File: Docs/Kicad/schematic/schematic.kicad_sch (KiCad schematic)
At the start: 35 parts

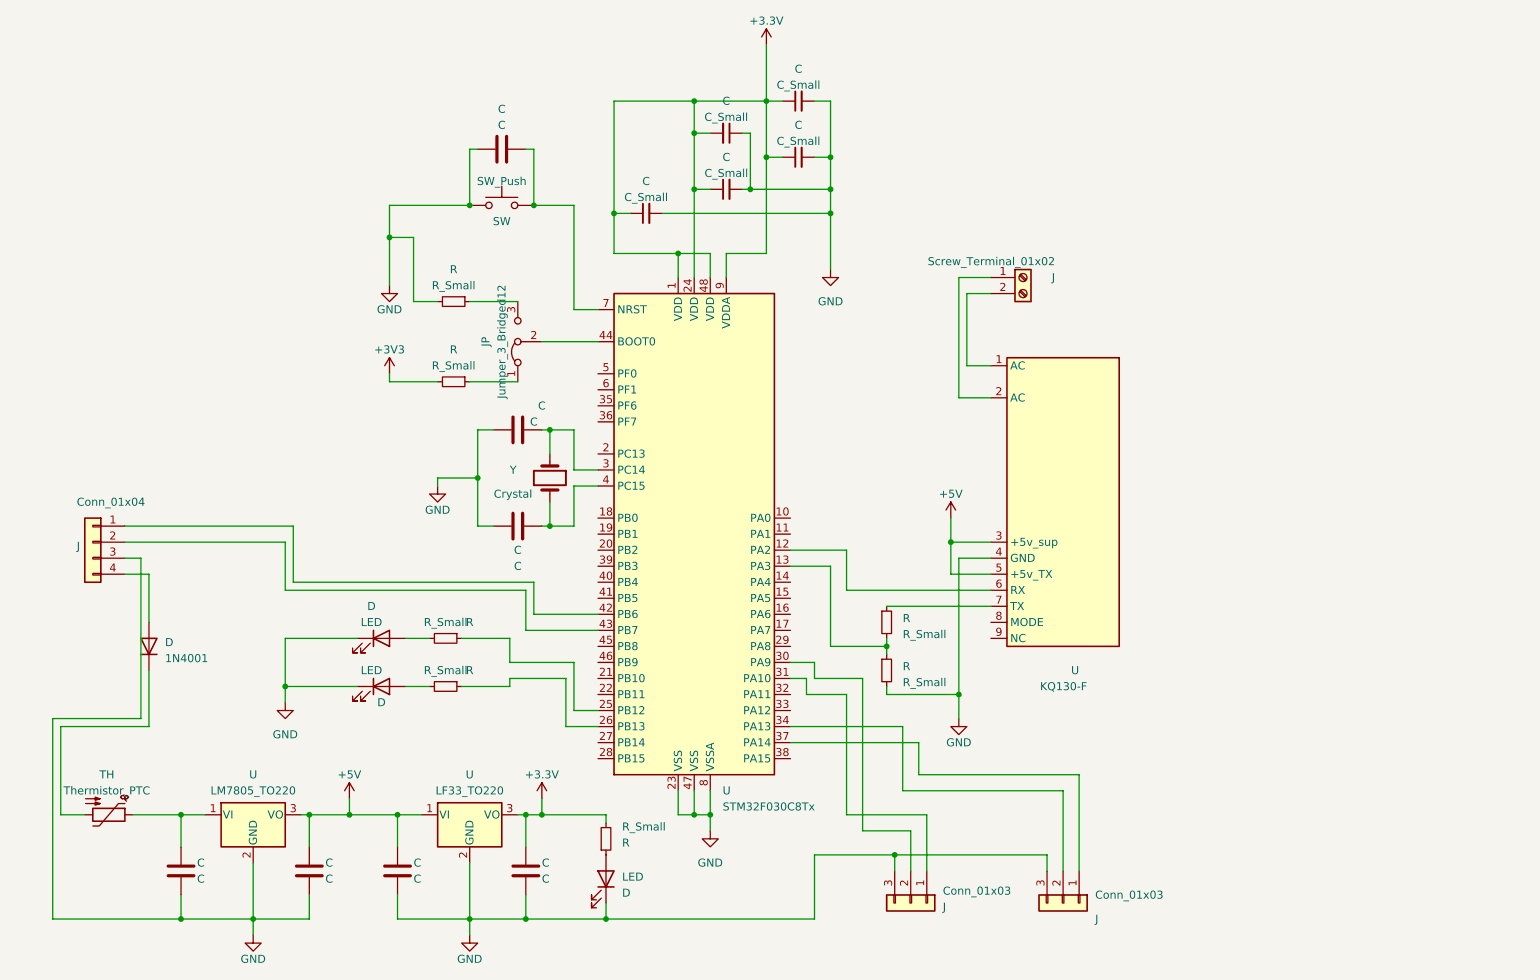
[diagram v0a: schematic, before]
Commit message: Schematic revisioned
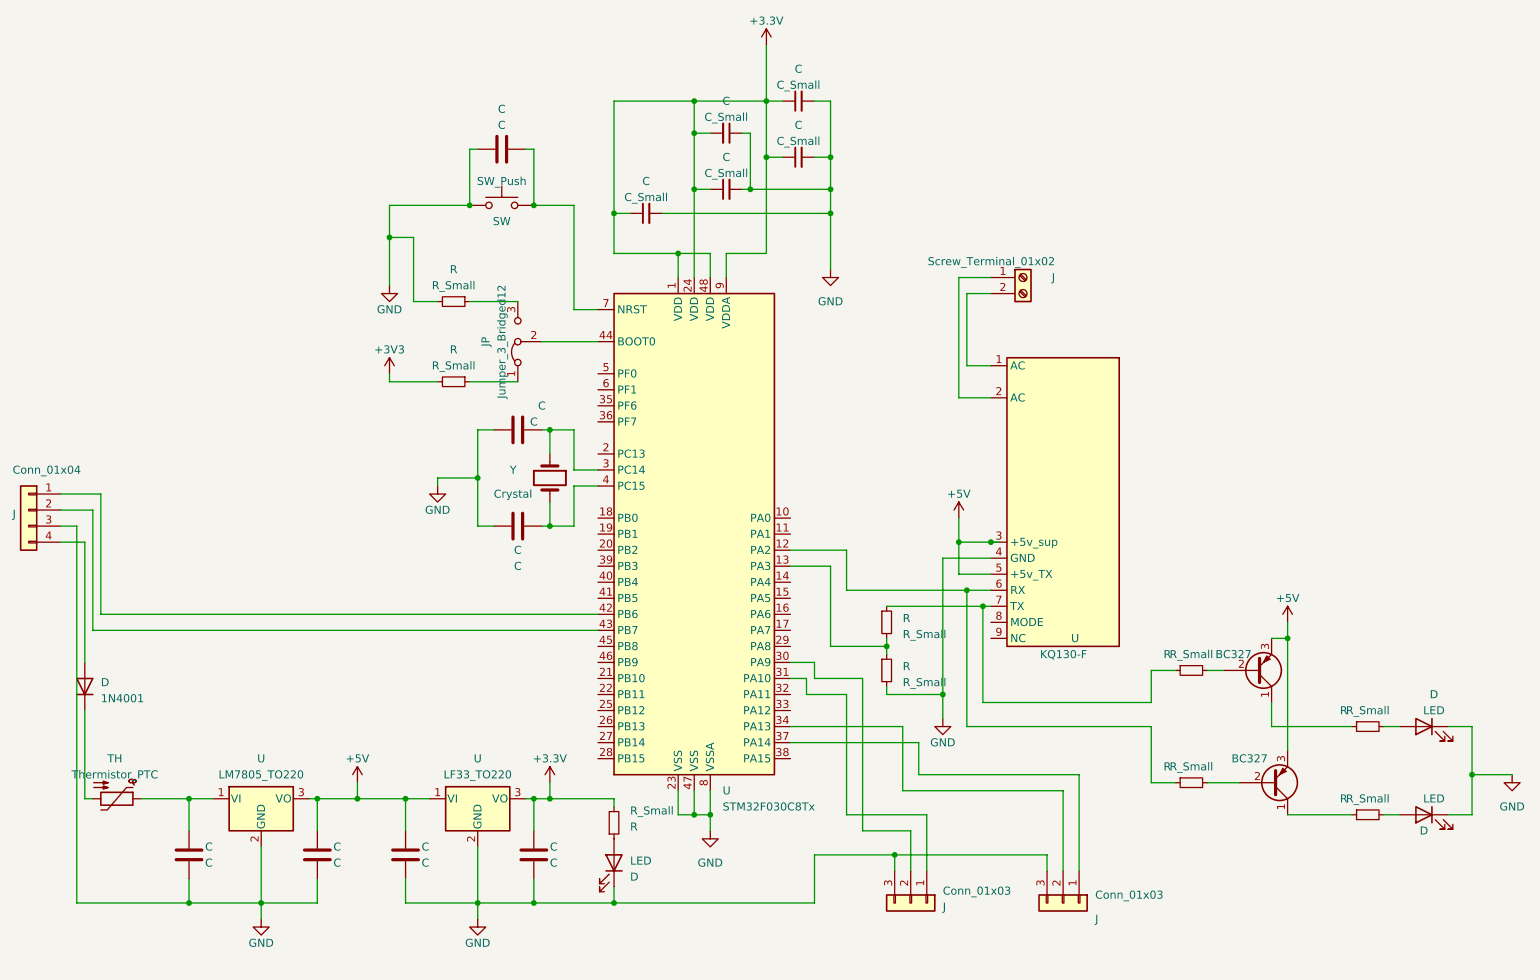
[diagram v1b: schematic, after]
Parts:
- removed C (x2): C, symbol Device:C
- added C (x2): C, symbol Device:C
- added Q (x2): BC327, Package_TO_SOT_THT:TO-92_Inline, symbol Transistor_BJT:BC327
- added R (x2): R_Small, symbol Device:R_Small
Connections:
- net +5V: now also C.1, Q.3 (E), Q.3 (E)
- net GND: now also C.2, C.2
- net at U.12 (PA2), U.6 (RX): now also R.1
- net at U.25 (PB12): no longer R.1
- net at U.26 (PB13): no longer R.1
- net at R.1, U.7 (TX): now also R.1
- net at TH.1, U.1 (VI): now also C.1
- new net: Q.1 (C), R.1 (x2)
- new net: Q.2 (B), R.2 (x2)
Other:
- moved on the sheet: C, D, J, R, TH, U
